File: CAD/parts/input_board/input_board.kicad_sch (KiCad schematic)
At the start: 19 parts, among them SW1 Power Switch, SW2 RST, SW3 BOOT Select, U1 NCV8114ASN330T1G, U3 STM32F042C6Ux

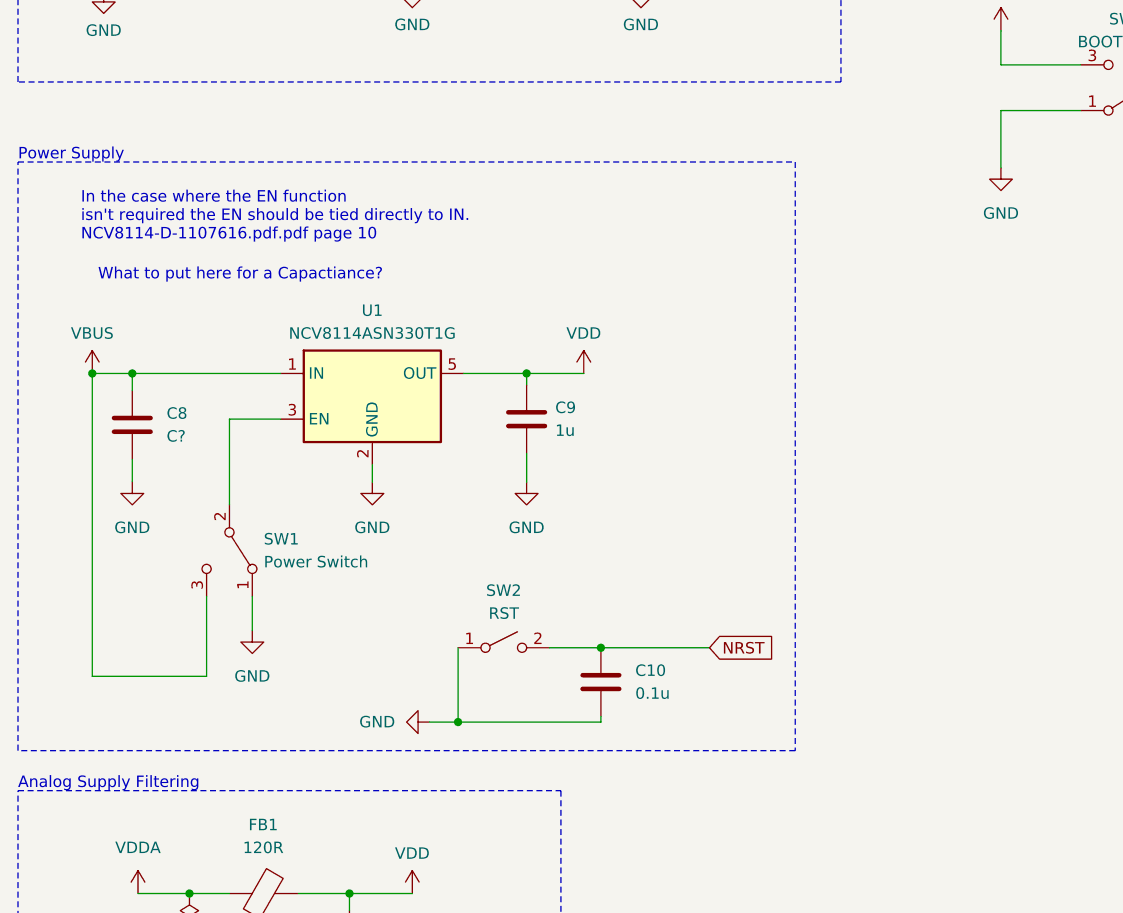
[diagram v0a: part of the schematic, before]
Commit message: hci pitch
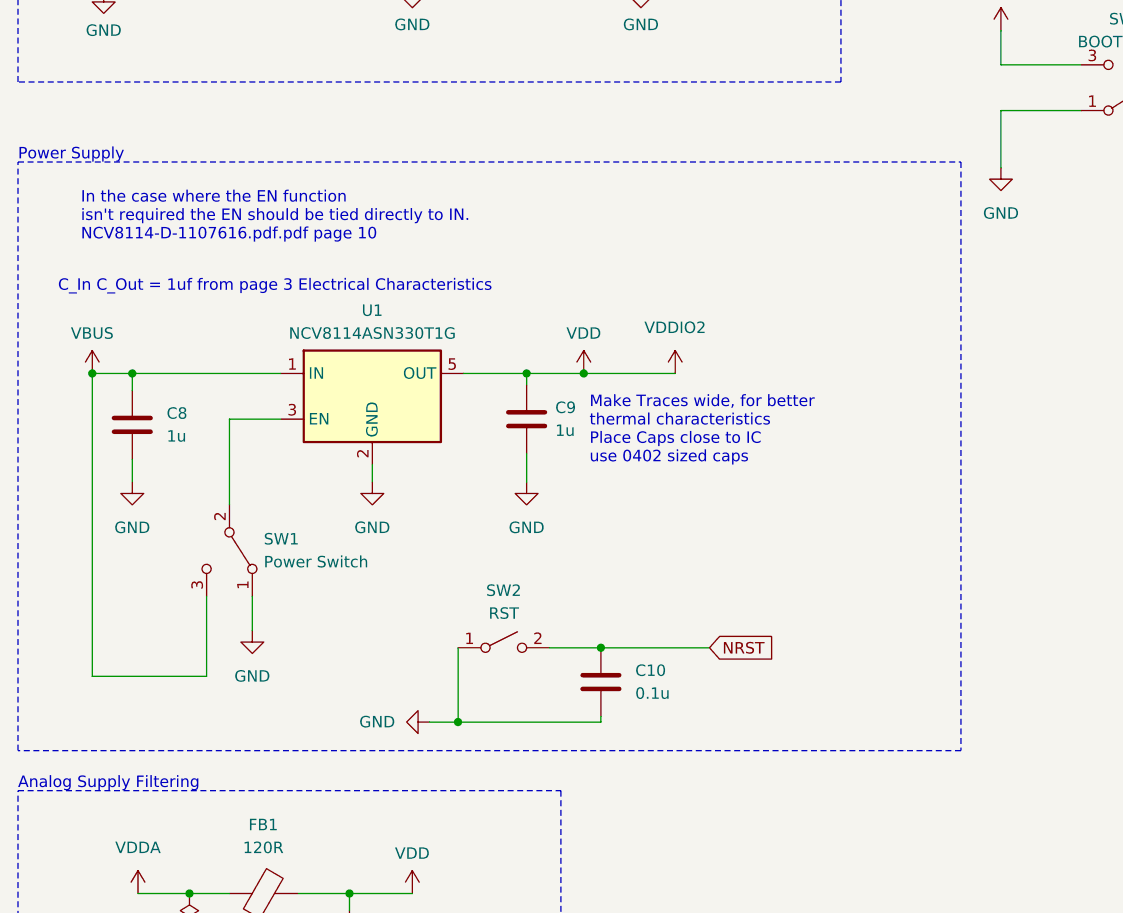
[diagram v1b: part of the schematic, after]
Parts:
- C8: value C? -> 1u
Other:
- note added: "C_In C_Out = 1uf from page 3 Electrical Characteristics"
- note added: "Make Traces wide, for better thermal characteristics Place Caps close to IC use 0402 sized caps"
- note removed: "What to put here for a Capactiance?"
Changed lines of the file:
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@@
   (junction (at 27.305 48.895) (diameter 0) (color 0 0 0 0)
+  )
+  (junction (at 80.645 92.71) (diameter 0) (color 0 0 0 0)
   )
   (junction (at 86.995 48.895) (diameter 0) (color 0 0 0 0)
@@
     (stroke (width 0) (type default))
   )
+  (wire (pts (xy 80.645 92.71) (xy 90.805 92.71))
+    (stroke (width 0) (type default))
+  )
   (wire (pts (xy 197.485 81.28) (xy 214.63 81.28))
     (stroke (width 0) (type default))
@@
     (fill (type none))
   )
-  (rectangle (start 17.78 69.215) (end 104.14 134.62)
+  (rectangle (start 17.78 69.215) (end 122.555 134.62)
     (stroke (width 0) (type dash))
     (fill (type none))
   )
+  (text "C_In C_Out = 1uf from page 3 Electrical Characteristics\n"
+    (at 22.225 83.82 0)
+    (effects (font (size 1.27 1.27)) (justify left bottom))
+  )
   (text "These Caps Need to be placed near the Pins on the PCB \n(either on same side, or on the other side!)\nstm32f048c6.pdf page 38\n"
     (at 22.86 30.48 0)
     (effects (font (size 1.27 1.27)) (justify left bottom))
   )
-  (text "What to put here for a Capactiance?" (at 26.67 82.55 0)
-    (effects (font (size 1.27 1.27)) (justify left bottom))
-  )
   (text "In the case where the EN function\nisn't required the EN should be tied directly to IN.\nNCV8114-D-1107616.pdf.pdf page 10"
     (at 24.765 78.105 0)
@@
   )
   (text "Power Supply" (at 17.78 69.215 0)
+    (effects (font (size 1.27 1.27)) (justify left bottom))
+  )
+  (text "Make Traces wide, for better\nthermal characteristics\nPlace Caps close to IC\nuse 0402 sized caps"
+    (at 81.28 102.87 0)
     (effects (font (size 1.27 1.27)) (justify left bottom))
   )
@@
     )
   )
+  (symbol (lib_id "power:VDDIO2") (at 90.805 92.71 0) (unit 1)
+    (in_bom yes) (on_board yes) (dnp no) (fields_autoplaced)
+    (property "Reference" "#PWR028" (at 90.805 96.52 0)
+      (effects (font (size 1.27 1.27)) hide)
+    )
+    (property "Value" "VDDIO2" (at 90.805 87.63 0)
+      (effects (font (size 1.27 1.27)))
+    )
+    (property "Footprint" "" (at 90.805 92.71 0)
+      (effects (font (size 1.27 1.27)) hide)
+    )
+    (property "Datasheet" "" (at 90.805 92.71 0)
+      (effects (font (size 1.27 1.27)) hide)
+    )
+    (pin "1")
+    (instances
+      (project "input_board"
+        (path "/0120ed21-7bf8-4cd4-88bf-009def744e7f"
+          (reference "#PWR028") (unit 1)
+        )
+      )
+    )
+  )
   (symbol (lib_id "power:VDDA") (at 184.785 42.545 0) (unit 1)
     (in_bom yes) (on_board yes) (dnp no)
@@
       (effects (font (size 1.27 1.27)) (justify left))
     )
-    (property "Value" "C?" (at 34.29 99.695 0)
-      (effects (font (size 1.27 1.27)) (justify left))
-    )
+    (property "Value" "1u" (at 34.29 99.695 0)
+      (effects (font (size 1.27 1.27)) (justify left))
+    )
